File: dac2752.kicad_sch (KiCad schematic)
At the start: 25 parts, among them U30 LTC2752B, U301 OPA2197D, U31 OPA2189DGK, U32 OPA2388DGK, U34 OPA2388DGK

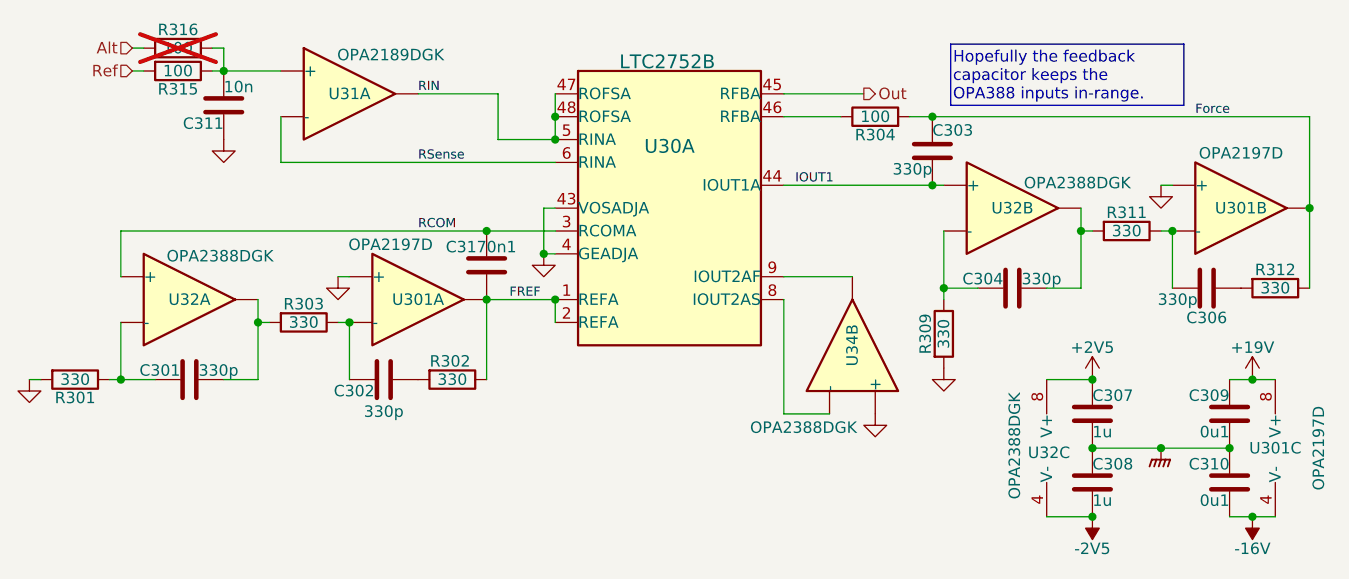
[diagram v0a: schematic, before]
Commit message: Front panel
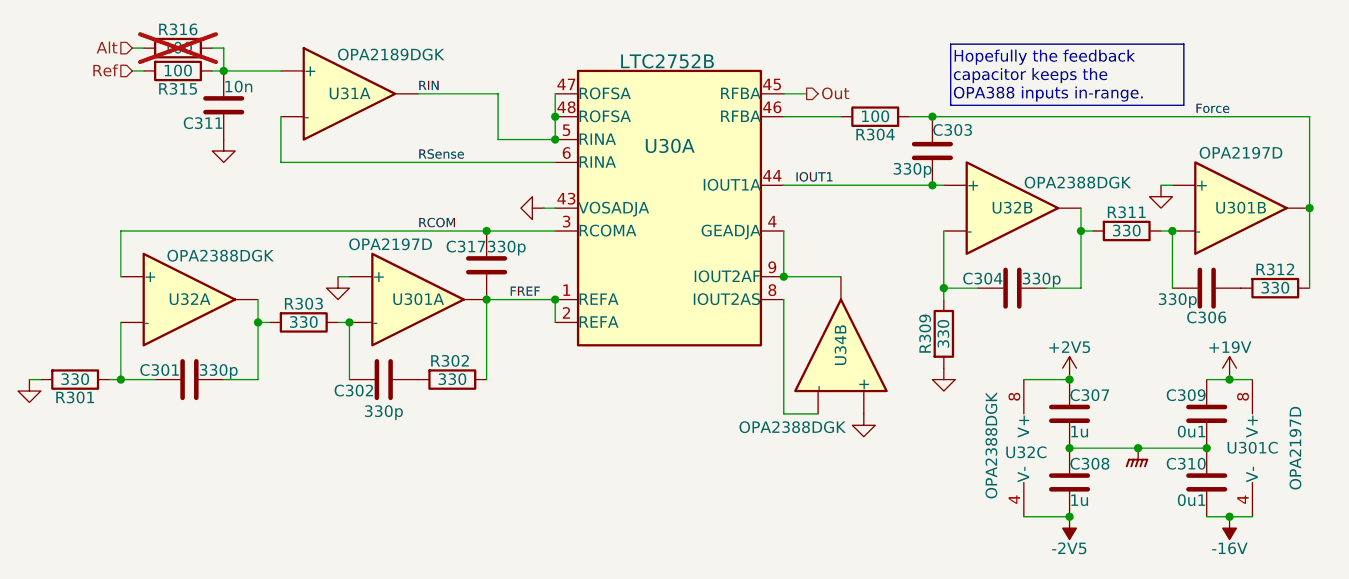
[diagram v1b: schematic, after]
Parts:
- C317: value 0n1 -> 330p; LCSC C14858 -> C1664
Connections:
- net GND: no longer U30.4 (GEADJA)
- net at U30.9 (IOUT2AF), U34.7: now also U30.4 (GEADJA)
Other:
- moved on the sheet: C307, C308, C309, C310, U301C, U32C, U34B
